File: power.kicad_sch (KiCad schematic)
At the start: 33 parts, among them J18 Conn_02x08_Odd_Even, J19 Conn_Coaxial, U12 TLV1117-33

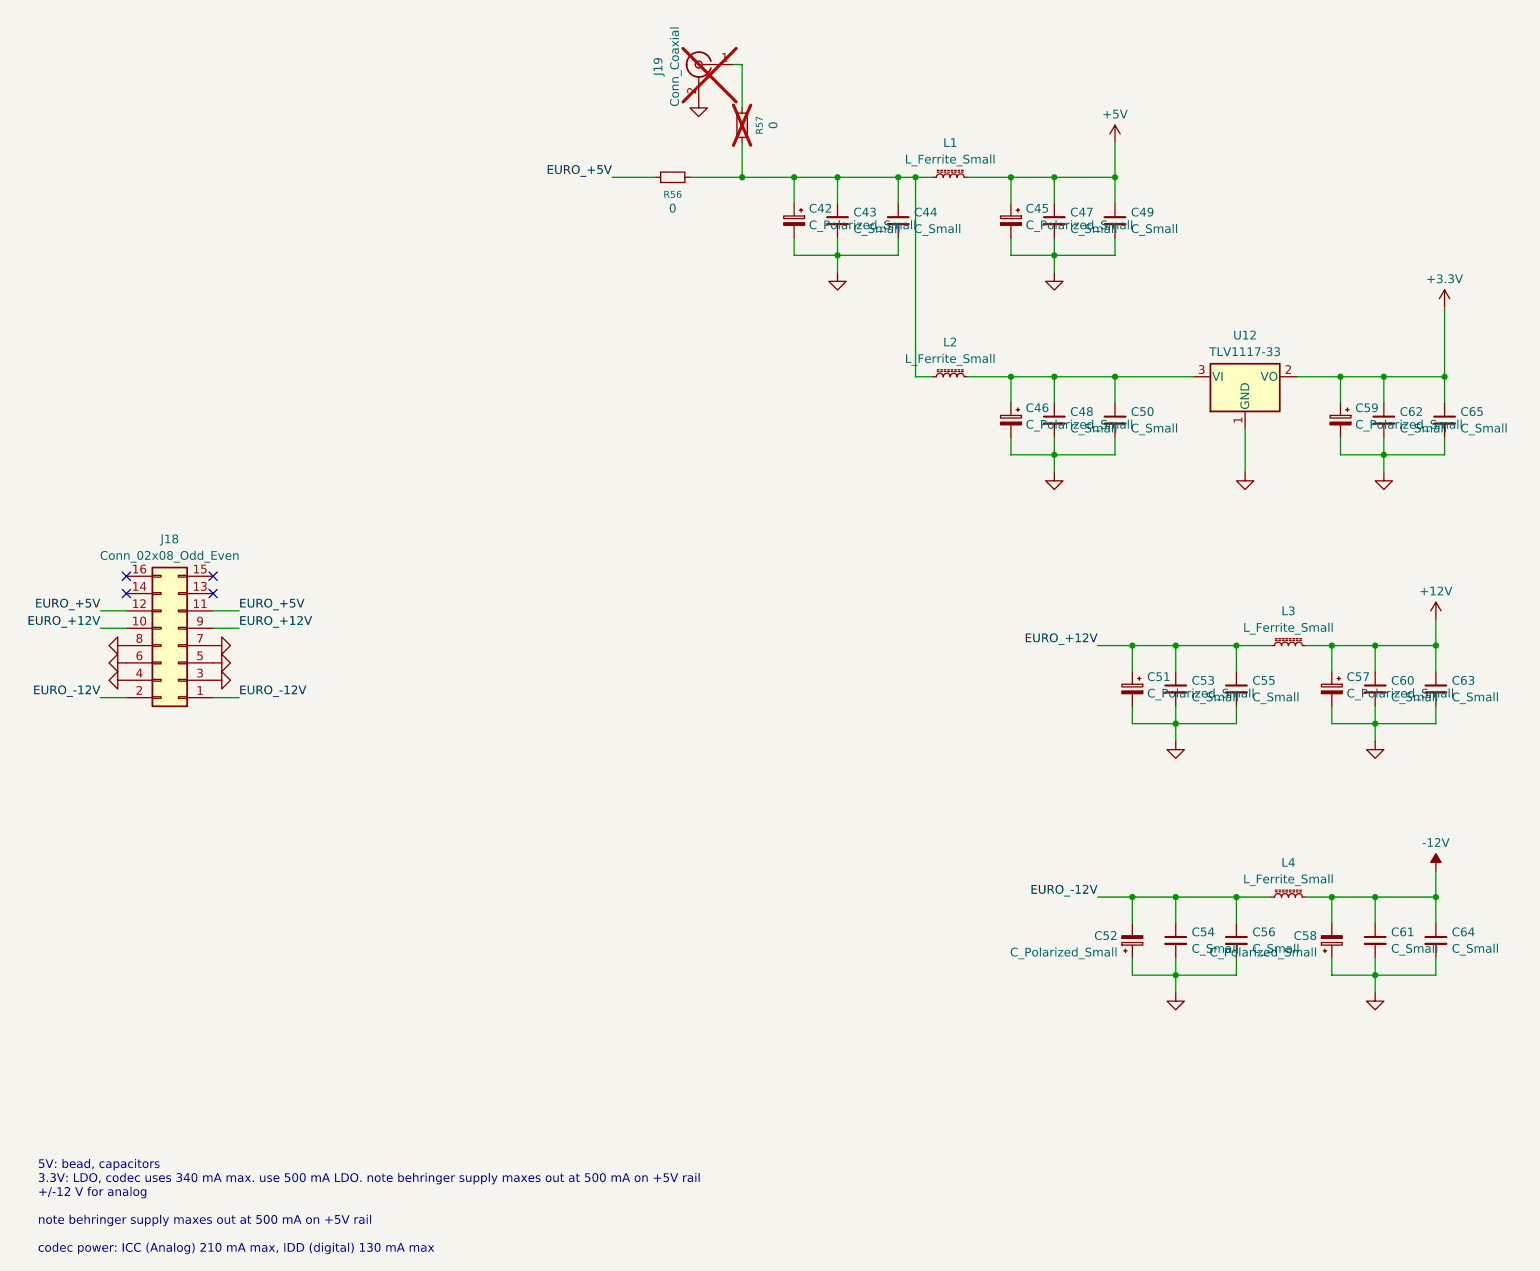
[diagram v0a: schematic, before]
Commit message: WIP layout
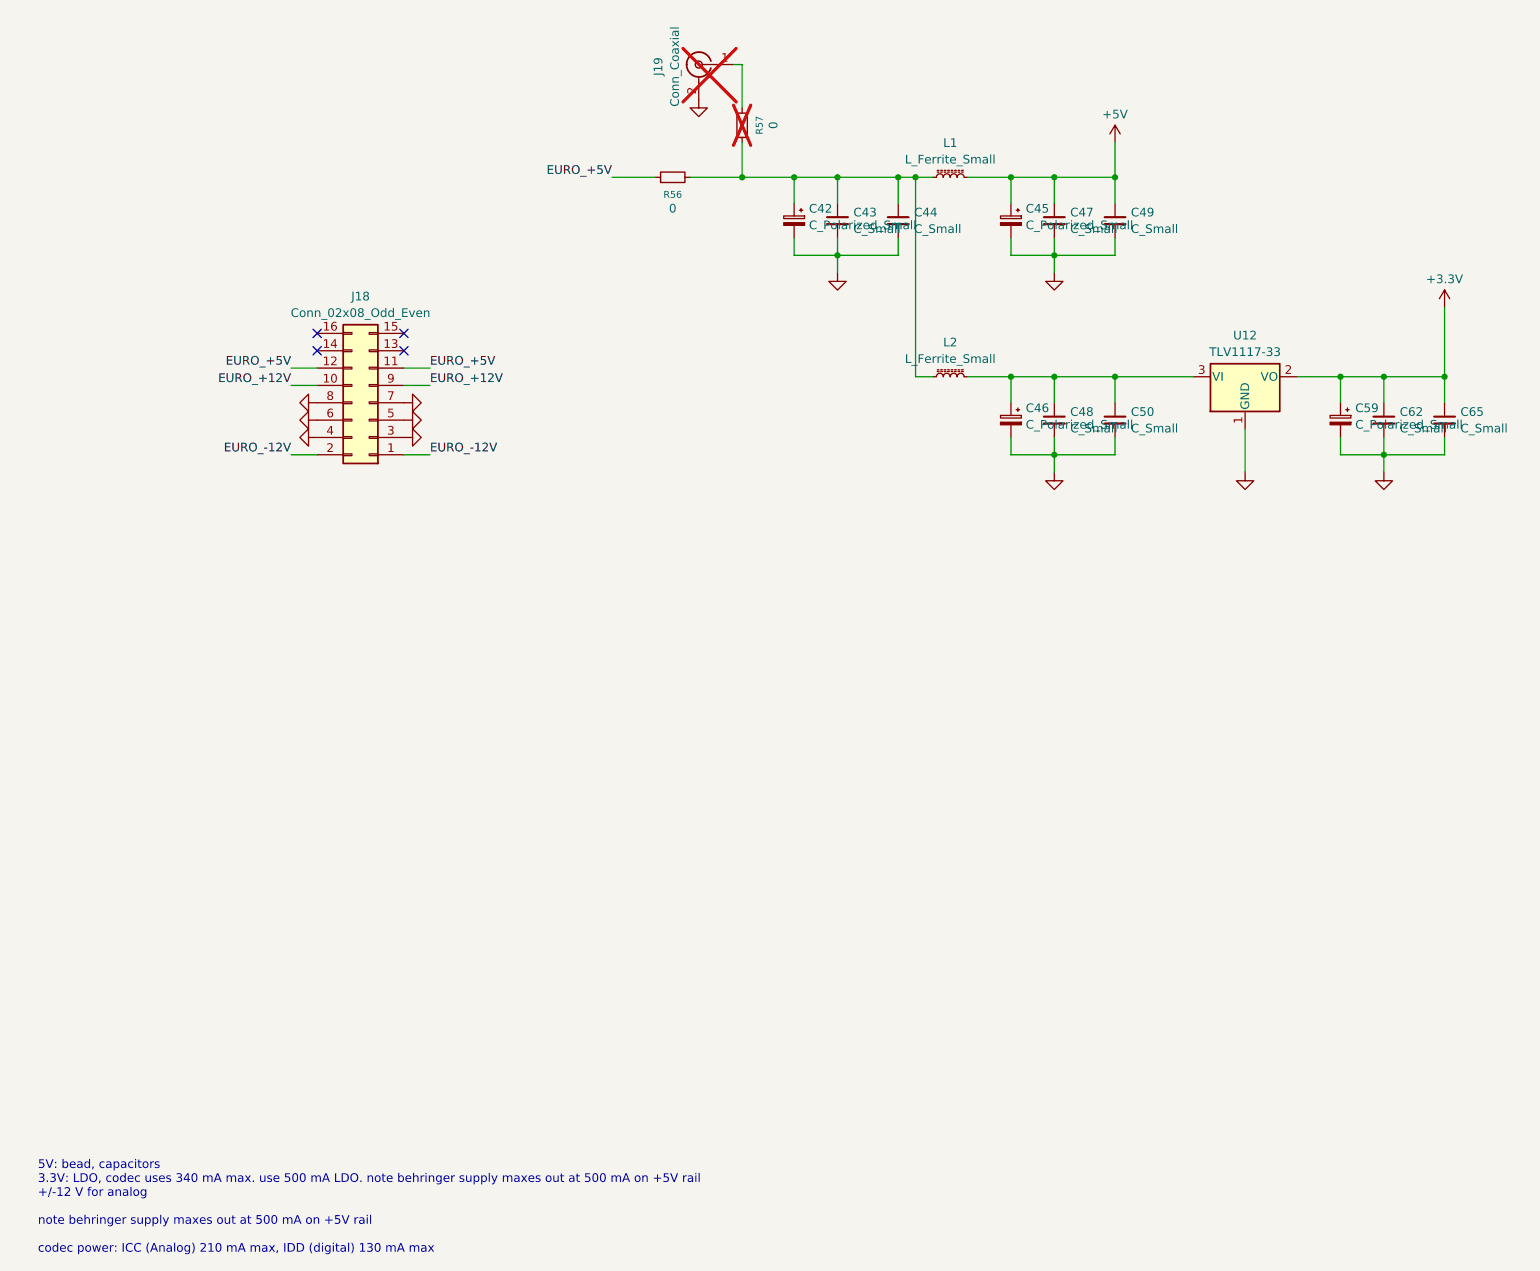
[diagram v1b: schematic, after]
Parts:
- removed C51, C52, C57, C58: C_Polarized_Small, Capacitor_THT:CP_Radial_D8.0mm_P3.50mm, symbol Device:C_Polarized_Small
- removed C53, C54, C55, C56, C60, C61, C63, C64: C_Small, Capacitor_SMD:C_0603_1608Metric, symbol Device:C_Small
- removed L3, L4: L_Ferrite_Small, Inductor_SMD:L_0603_1608Metric, symbol Device:L_Ferrite_Small
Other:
- moved on the sheet: J18
